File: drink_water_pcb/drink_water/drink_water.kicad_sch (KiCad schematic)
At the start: 47 parts, among them J1 Conn_01x04, J2 USB_C_Receptacle_USB2.0_16P, J3 Conn_01x02, J4 Conn_01x02, Q1 FS8205, SW1 SW_SPDT, U1 ESP32-C3-WROOM-02, U2 USBLC6-2SC6, U3 TP4056, U4 DW01A, U5 LSM6DSM, U6 FDC1004, U7 AMS1117-3.3

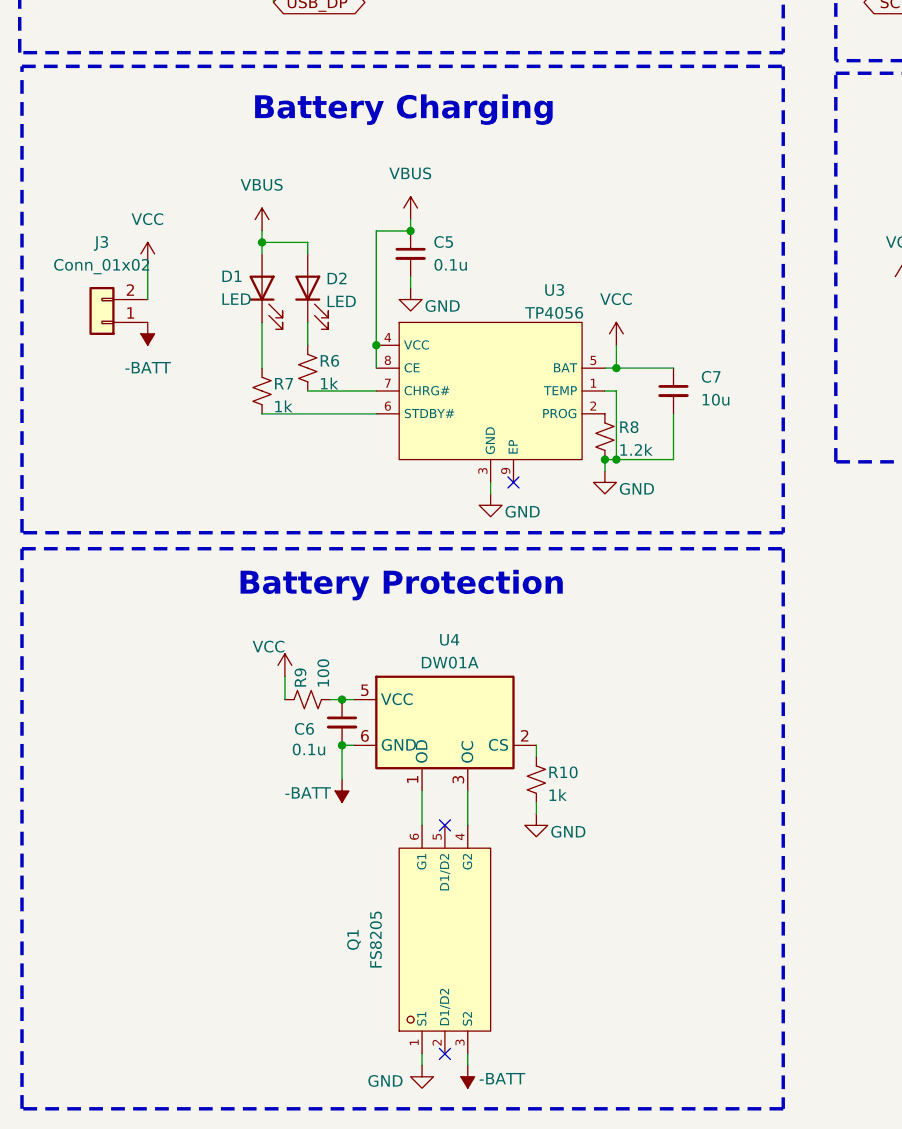
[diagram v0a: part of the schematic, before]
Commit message: Initial layout, pre-route
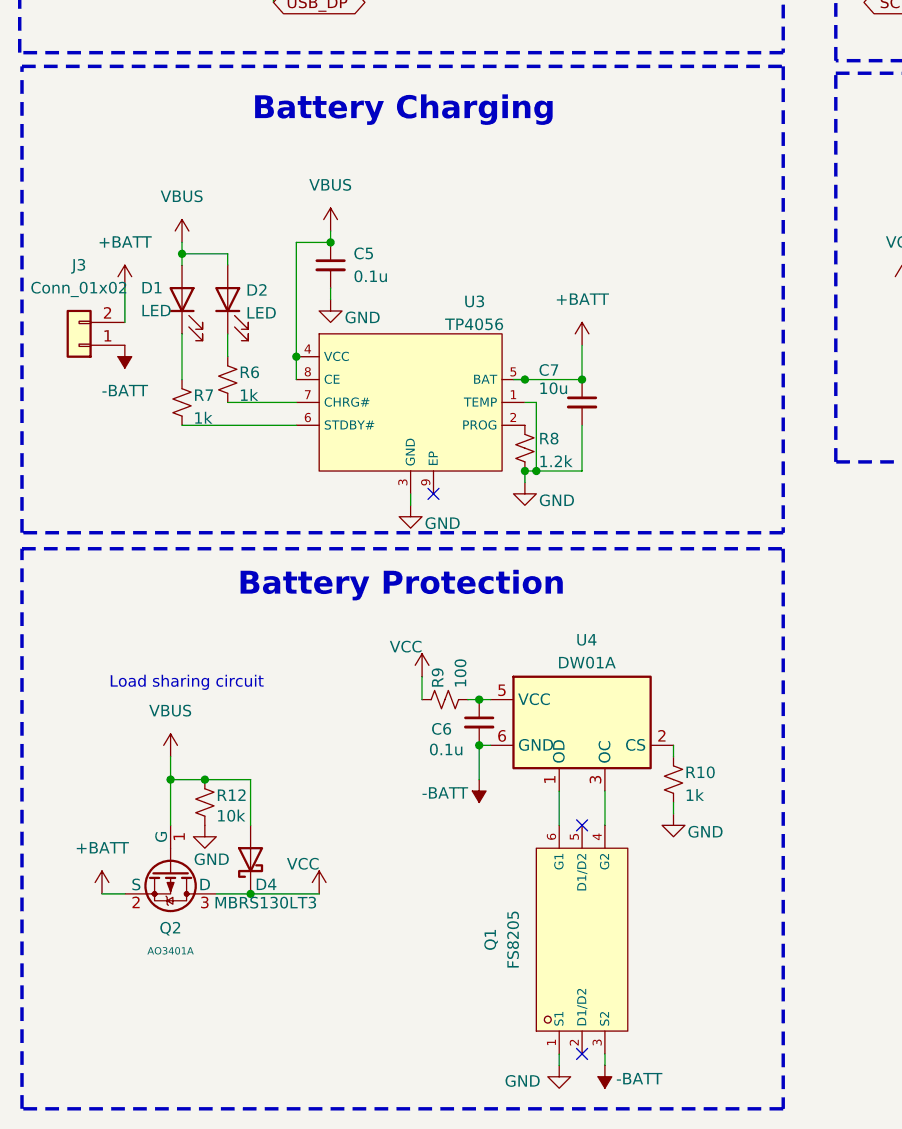
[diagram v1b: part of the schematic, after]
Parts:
- added D4: MBRS130LT3, Diode_SMD:D_SMB, symbol Device:D_Schottky
- added Q2: AO3401A, Package_TO_SOT_SMD:SOT-23, symbol JLCPCB-Transistors:PMOS,AO3401A
- added R12: 10k, Resistor_SMD:R_0402_1005Metric, symbol Device:R_Small_US
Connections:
- net GND: now also R12.2
- net VBUS: now also D4.2 (A), Q2.1 (G), R12.1
- net VCC: now also D4.1 (K), Q2.3 (D); no longer C7.1, J3.2 (Pin_2), U3.5 (BAT)
- new net +BATT: C7.1, J3.2 (Pin_2), Q2.2 (S), U3.5 (BAT)
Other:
- note added: "Load sharing circuit"
- moved on the sheet: C5, C6, C7, D1, D2, J3, Q1, R10, R6, R7, R8, R9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
